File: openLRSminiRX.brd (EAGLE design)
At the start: 20.2 x 21.8 mm, 19 parts, among them U1 ATMEGA328P, U2 V_REG_LDOSMD

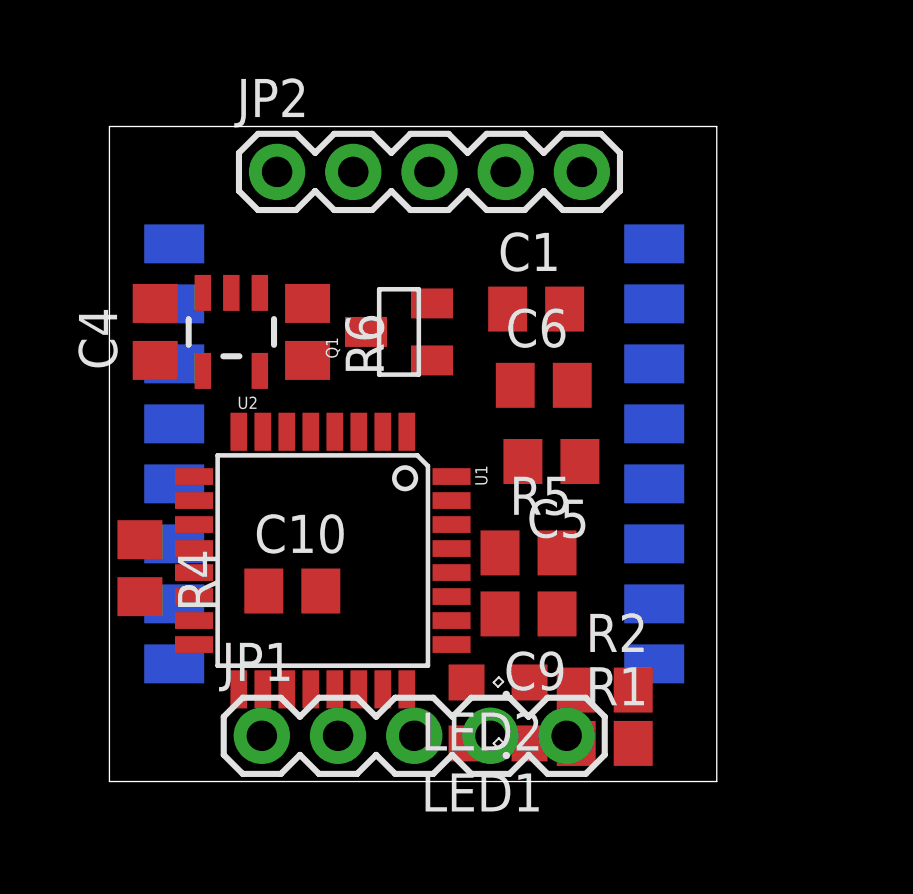
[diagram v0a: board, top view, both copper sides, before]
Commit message: update, fully routed.
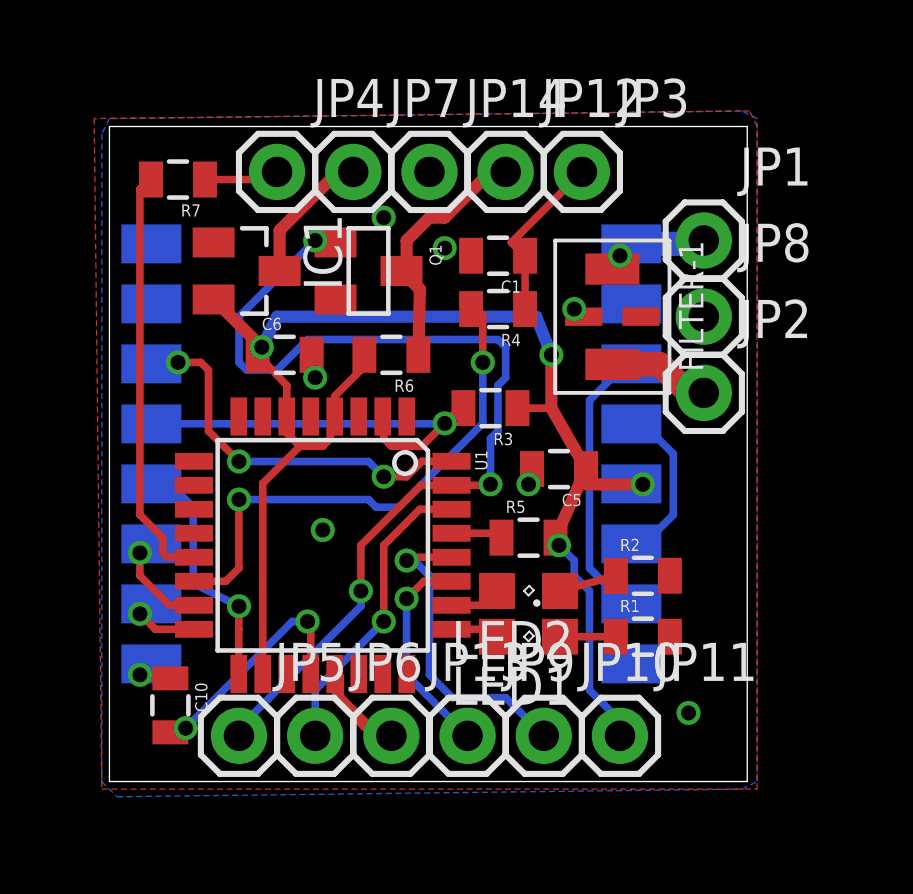
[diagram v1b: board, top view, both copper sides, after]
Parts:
- removed C4, C9: (no value), rcl:C0805
- removed U2: V_REG_LDOSMD, SparkFun-PowerIC:SOT23-5
- added FILTER-1: LFCN-490, minicircuits:FV1206
- added IC1: MCP1703CB, linear:SOT23
- added JP10: SCL, SparkFun-Connectors:1X01
- added JP11: VCC, SparkFun-Connectors:1X01
- added JP12: SBUS, SparkFun-Connectors:1X01
- added JP13, JP14, JP8: GND, SparkFun-Connectors:1X01
- added JP3: RSSI, SparkFun-Connectors:1X01
- added JP4: PPM, SparkFun-Connectors:1X01
- added JP5: TXD, SparkFun-Connectors:1X01
- added JP6: RXD, SparkFun-Connectors:1X01
- added JP7: VIN, SparkFun-Connectors:1X01
- added JP9: SDA, SparkFun-Connectors:1X01
- added R3, R7: (no value), SparkFun-Resistors:0805
- C1, C10, C5, C6: device rcl:C0805 -> SparkFun-Capacitors:0805
- JP1: value (none) -> ANT; device SparkFun-Connectors:1X05 -> SparkFun-Connectors:1X01
- JP2: value (none) -> ANTF; device SparkFun-Connectors:1X05 -> SparkFun-Connectors:1X01
- R1, R2, R4, R5, R6: device rcl:R0805 -> SparkFun-Resistors:0805
- moved JP1 22.1 mm to (19.8, 18.0)
- moved JP2 16.0 mm to (19.8, 13.0)
- moved R4 14.7 mm to (13.0, 15.7), turned to 180 degrees
- moved C6 8.70 mm to (5.84, 14.2)
- moved C10 5.57 mm to (2.03, 2.54), turned to 270 degrees
- moved R2 4.02 mm to (17.8, 6.86)
- moved R1 3.78 mm to (17.8, 4.83)
- moved LED1 3.70 mm to (14.0, 4.83)
- moved LED2 3.21 mm to (14.0, 6.35)
- moved R6 2.90 mm to (9.40, 14.2), turned to 180 degrees
- moved Q1 2.27 mm to (8.64, 17.0), turned to 270 degrees
- moved C1 2.18 mm to (13.0, 17.5), turned to 180 degrees
- moved U$1 0.76 mm to (9.40, 10.9)
- moved R5 0.51 mm to (14.0, 8.13)
- moved U1 0.51 mm to (7.11, 7.87)
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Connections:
- removed net DTR: C9.1
- removed net N$16: C4.1, U2.4
- new net N$1: FILTER-1.1, JP1.1, U$1.1
- new net N$4: FILTER-1.3, JP2.1
- new net N$5: JP4.1, R7.1
- net GND: now also FILTER-1.2, FILTER-1.4, JP13.1, JP14.1, JP8.1; no longer C4.2, U2.2
- net N$10: now also R3.2
- net N$18: no longer C9.2
- net PPM: now also R7.2
- net RSSI: now also JP3.1
- net RXD: now also JP6.1
- net SBUS: now also JP12.1
- net SCL: now also JP10.1; no longer JP2.2
- net SDA: now also JP9.1; no longer JP2.3
- net TXD: now also JP5.1
- net VCC: now also IC1.2, JP11.1, R3.1; no longer JP2.1, U2.5
- net VIN: now also IC1.3, JP7.1; no longer U2.1, U2.3
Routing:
- net VCC: track 0.00 -> 48.1 mm, vias 0 -> 4
- net TXD: track 0.00 -> 33.4 mm, vias 0 -> 3
- net N$17: track 0.00 -> 17.4 mm, vias 0 -> 2
- net N$10: track 0.00 -> 14.6 mm, vias 0 -> 1
- net PPM: track 0.00 -> 14.0 mm
- net N$11: track 0.00 -> 13.0 mm, vias 0 -> 3
- net SCL: track 0.00 -> 10.5 mm, vias 0 -> 1
- net RXD: track 0.00 -> 10.1 mm, vias 0 -> 1
- net N$3: track 0.00 -> 9.38 mm
- net SBUS: track 0.00 -> 8.38 mm
- net N$9: track 0.00 -> 8.22 mm, vias 0 -> 1
- net N$19: track 0.00 -> 7.89 mm, vias 0 -> 2
- net SDA: track 0.00 -> 7.15 mm, vias 0 -> 1
- net RSSI: track 0.00 -> 5.74 mm
- net N$2: track 0.00 -> 5.64 mm
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- added copper zone on layer 1, net GND
- added copper zone on layer 16, net GND
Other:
- board size 20.2 x 21.8 mm -> 21.3 x 21.8 mm
